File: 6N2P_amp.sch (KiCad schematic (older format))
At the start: 78 parts, among them J1 guitar_in, J2 speaker, J3 fx_send, J4 fx_return, U1 ECC83, U2 ECC83, U3 6N1P, U4 DSN-MINI-360, U5 DSN-MINI-360, U6 DSN-MINI-360, U7 NCH6100HV

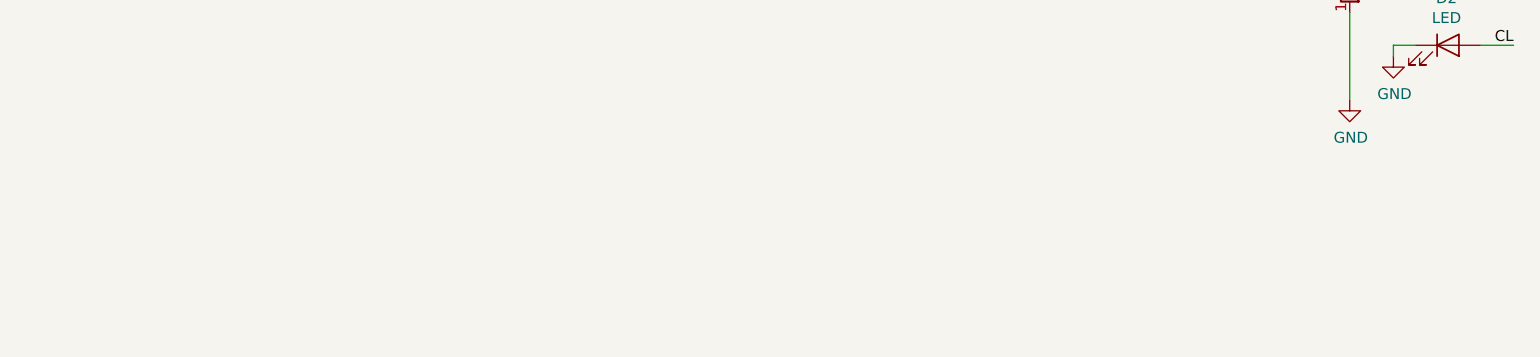
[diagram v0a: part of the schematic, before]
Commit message: snap
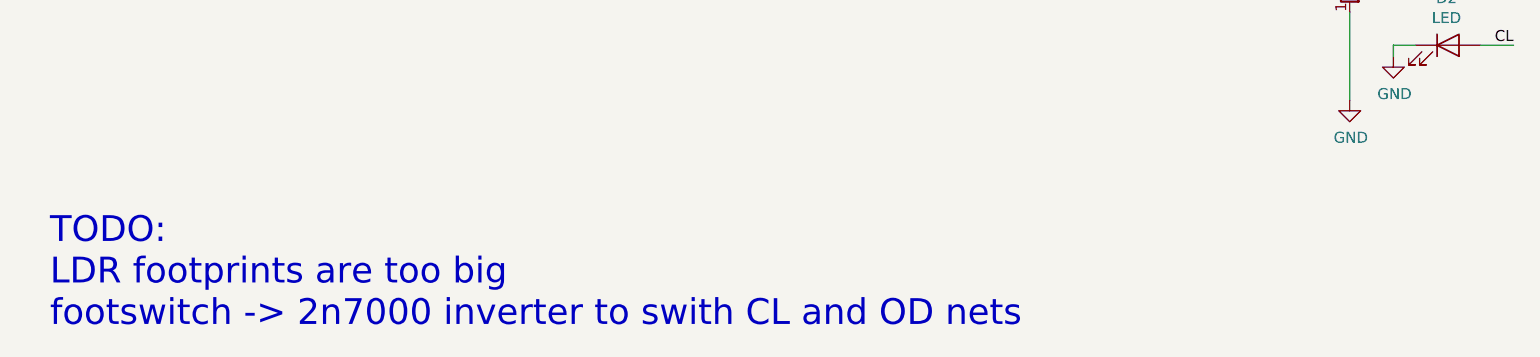
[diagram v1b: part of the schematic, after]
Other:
- note added: "TODO:\nLDR footprints are too big\nfootswitch -> 2n7000 inverter to swith CL and OD nets"
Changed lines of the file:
@@
 Wire Wire Line
 	12900 8500 12900 8450
+Text Notes 1550 13600 0    118  ~ 0
+TODO:\nLDR footprints are too big\nfootswitch -> 2n7000 inverter to swith CL and OD nets
 $EndSCHEMATC
